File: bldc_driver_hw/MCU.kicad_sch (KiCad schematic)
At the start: 16 parts, among them U9 STM32G474RETx, Y1 Crystal

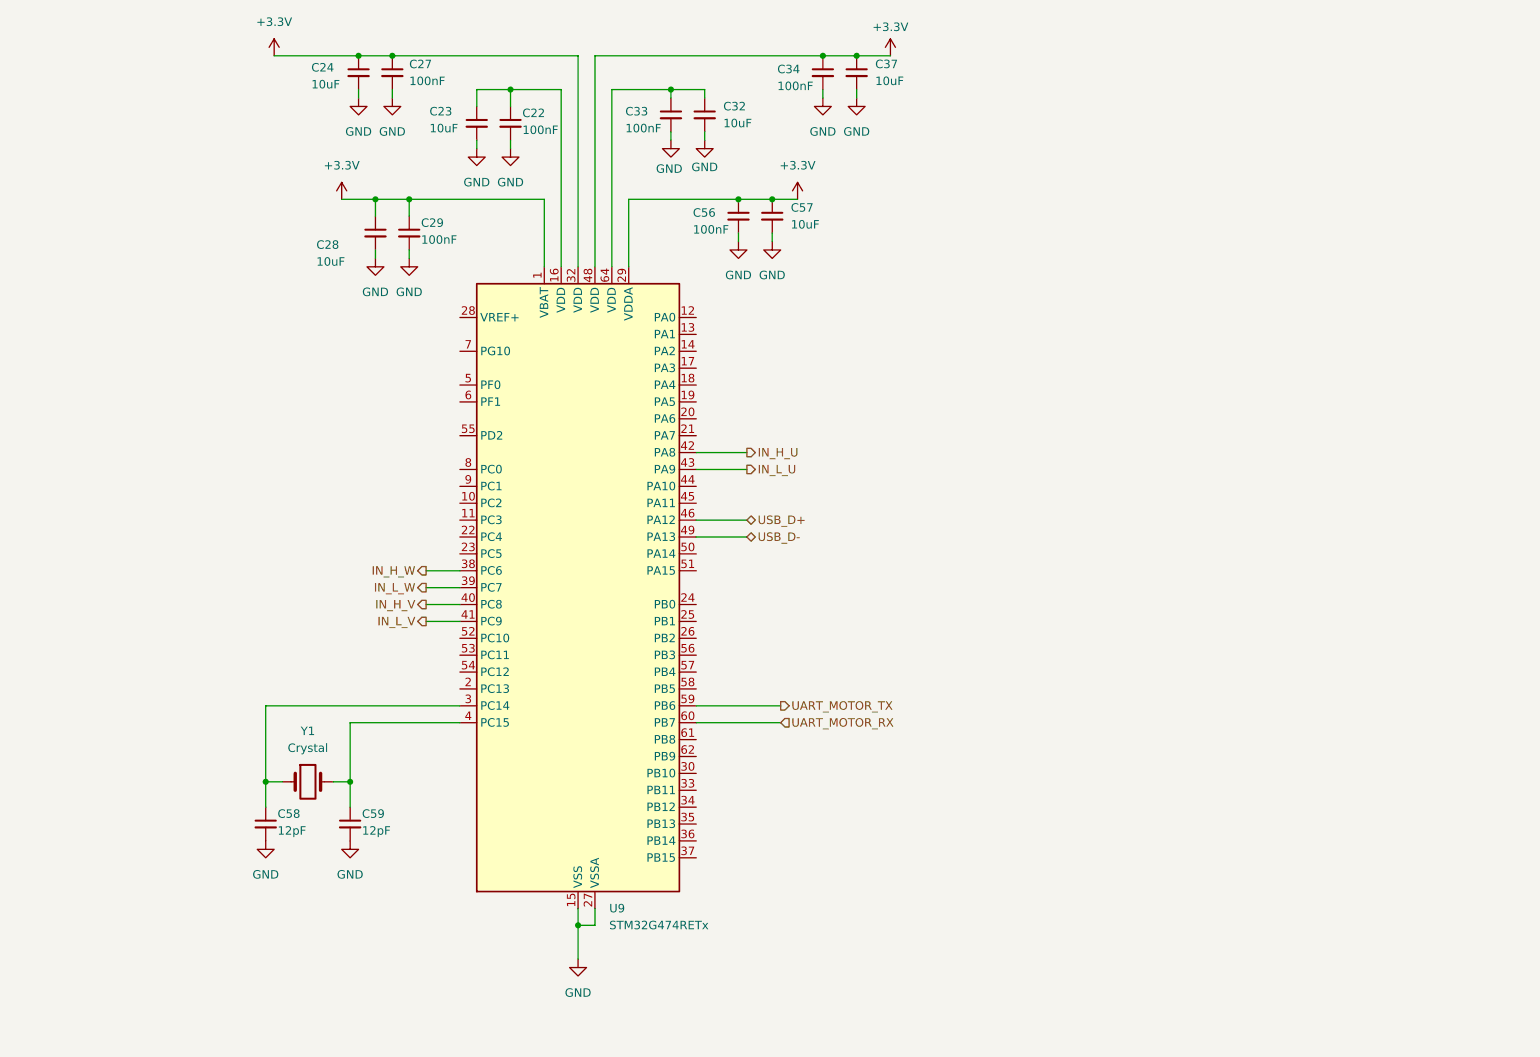
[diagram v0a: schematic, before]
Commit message: wip
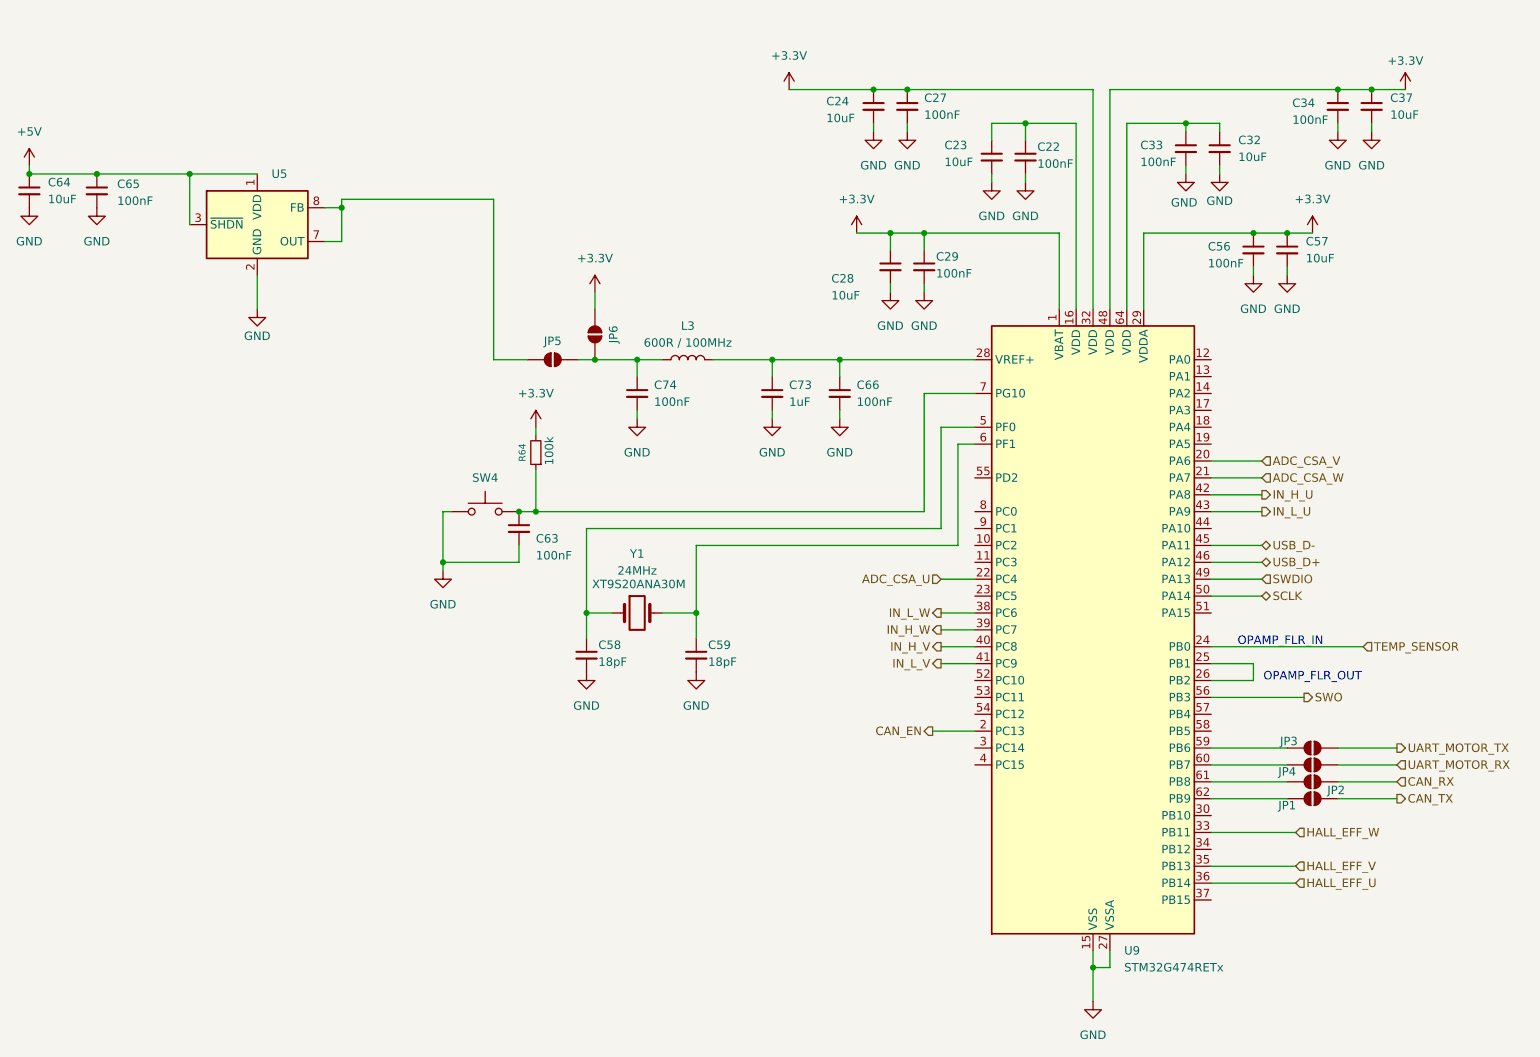
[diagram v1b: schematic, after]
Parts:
- added C63, C65, C66, C74: 100nF, Capacitor_SMD:C_0603_1608Metric, symbol Device:C_Small
- added C64: 10uF, Capacitor_SMD:C_0603_1608Metric, symbol Device:C_Small
- added C73: 1uF, Capacitor_SMD:C_0603_1608Metric, symbol Device:C_Small
- added JP1, JP2, JP3, JP4, JP5, JP6: SolderJumper_2_Open, Jumper:SolderJumper-2_P1.3mm_Open_RoundedPad1.0x1.5mm, symbol Jumper:SolderJumper_2_Open
- added L3: 600R / 100MHz, Resistor_SMD:R_1206_3216Metric, symbol Device:L
- added R64: 100k, Resistor_SMD:R_0805_2012Metric, symbol Device:R_Small
- added SW4: SW_Push, symbol Switch:SW_Push
- added U5: MCP1501-33xSN, Package_SO:SOIC-8_3.9x4.9mm_P1.27mm, symbol Reference_Voltage:MCP1501-33xSN
- C58, C59: value 12pF -> 18pF
- Y1: value Crystal -> 24MHz; footprint (none) -> Crystal:Crystal_HC49-U_Vertical
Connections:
- net +3.3V: now also JP6.1 (A), R64.2
- net GND: now also C63.2, C64.2, C65.2, C66.2, C73.2, C74.2, SW4.1, U5.2 (GND), U5.4 (GND), U5.5 (GND), U5.6 (GND)
- net IN_H_W: now also U9.39 (PC7); no longer U9.38 (PC6)
- net IN_L_W: now also U9.38 (PC6); no longer U9.39 (PC7)
- net UART_MOTOR_RX: now also JP4.2 (B); no longer U9.60 (PB7)
- net UART_MOTOR_TX: now also JP3.2 (B); no longer U9.59 (PB6)
- net USB_D-: now also U9.45 (PA11); no longer U9.49 (PA13)
- net at C59.1, Y1.2: now also U9.6 (PF1); no longer U9.4 (PC15)
- net at C58.1, Y1.1: now also U9.5 (PF0); no longer U9.3 (PC14)
- net CAN_EN: now reaches U9.2 (PC13)
- net ADC_CSA_V: now reaches U9.20 (PA6)
- net ADC_CSA_W: now reaches U9.21 (PA7)
- net ADC_CSA_U: now reaches U9.22 (PC4)
- net TEMP_SENSOR: now reaches U9.24 (PB0)
- net at U9.25 (PB1): now also U9.26 (PB2)
- net at U9.28 (VREF+): now also C66.1, C73.1, L3.2
- net HALL_EFF_W: now reaches U9.33 (PB11)
- net HALL_EFF_V: now reaches U9.35 (PB13)
- net HALL_EFF_U: now reaches U9.36 (PB14)
- net SCLK: now reaches U9.50 (PA14)
- net SWO: now reaches U9.56 (PB3)
- net at U9.61 (PB8): now also JP2.1 (A)
- net at U9.62 (PB9): now also JP1.1 (A)
- net at U9.7 (PG10): now also C63.1, R64.1, SW4.2
- new net: JP5.1 (A), U5.7 (OUT), U5.8 (FB)
- new net: C74.1, JP5.2 (B), JP6.2 (B), L3.1
- new net: JP3.1 (A), U9.59 (PB6)
- new net: JP4.1 (A), U9.60 (PB7)
- new net +5V: C64.1, C65.1, U5.1 (VDD), U5.3 (~{SHDN})
- new net CAN_RX: JP2.2 (B)
- new net CAN_TX: JP1.2 (B)
- new net SWDIO: U9.49 (PA13)
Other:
- note added: "OPAMP_FLR_IN"
- note added: "OPAMP_FLR_OUT"
- moved on the sheet: C22, C23, C24, C27, C28, C29, C32, C33, C34, C37, C56, C57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
